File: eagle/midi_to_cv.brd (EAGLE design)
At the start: 100 x 80 mm, 57 parts, among them Q3 2N3904, Q4 2N3904, Q5 2N3904, Q6 2SK30, U1 ATMEGA328P_PDIP

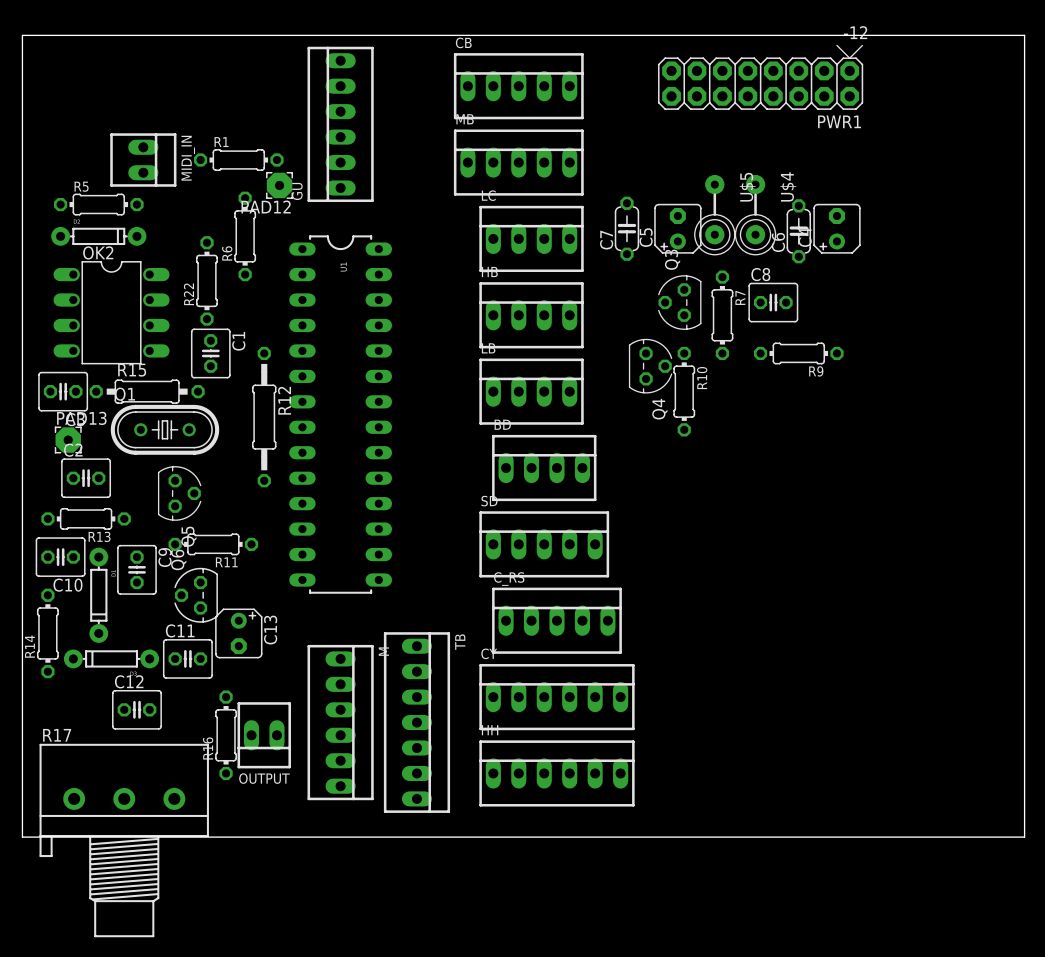
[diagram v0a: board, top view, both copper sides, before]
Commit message: 95pct auto
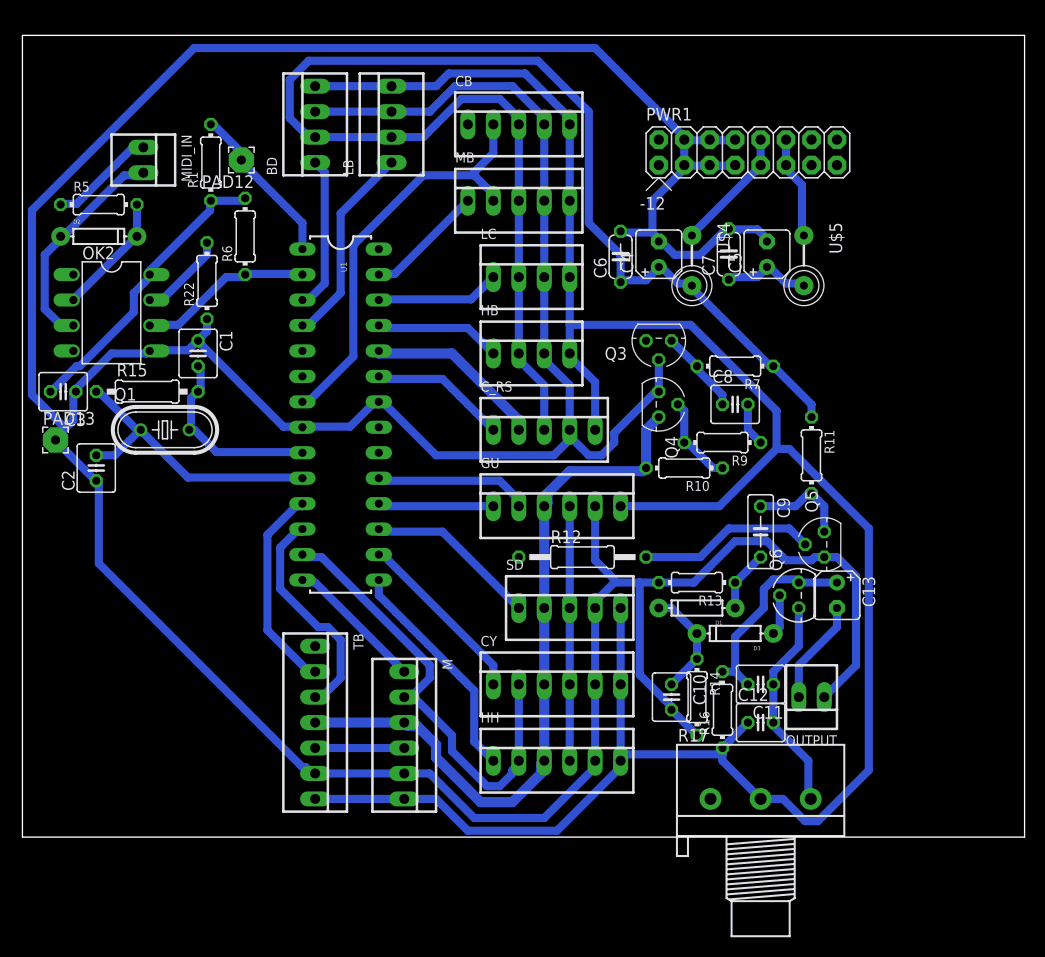
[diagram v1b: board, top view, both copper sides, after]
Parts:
- C9: device rcl:C025-040X050 -> rcl:C050-025X075
- moved R14 65.1 mm to (67.3, 14.0), turned to 270 degrees
- moved Q5 65.0 mm to (80.0, 29.2), turned to 90 degrees
- moved R17 63.5 mm to (73.7, 3.81)
- moved C10 62.5 mm to (64.8, 14.0), turned to 270 degrees
- moved C9 62.3 mm to (73.7, 30.5)
- moved D3 62.3 mm to (71.1, 20.3)
- moved C12 62.2 mm to (73.7, 11.4)
- moved R13 61.3 mm to (67.3, 25.4)
- moved R11 60.3 mm to (78.7, 38.1), turned to 270 degrees
- moved C13 59.8 mm to (81.3, 24.1)
- moved D1 59.7 mm to (67.3, 22.9), turned to 180 degrees
- moved Q6 59.7 mm to (77.5, 24.1)
- moved C11 57.2 mm to (73.7, 15.2), turned to 180 degrees
- moved OUTPUT 54.7 mm to (78.7, 14.0)
- moved R16 49.6 mm to (69.8, 12.7)
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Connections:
- removed net GU_LONG: GU.1, U1.3
- removed net GU_SHORT: GU.2, U1.4
- new net N$10: GU.2, U1.19
- new net N$9: GU.1, U1.18
- net ACCENT: now also U1.28; no longer U1.5
- net CB_TRIG: now also U1.5; no longer U1.28
- net CY_KILL: now also U1.13; no longer U1.14
- net C_TRIG: now also U1.24; no longer U1.18
- net M_TRIG: now also U1.14; no longer U1.13
- net N$3: now also U1.3; no longer U1.23
- net N$7: now also U1.4; no longer U1.24
- net RS_TRIG: now also U1.23; no longer U1.17
- net SD_TRIG: now also U1.17; no longer U1.19
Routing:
- net GND: track 0.00 -> 442.4 mm
- net RETURN: track 0.00 -> 227.4 mm
- net +12V: track 0.00 -> 174.4 mm
- net +5V: track 0.00 -> 80.8 mm
- net NOISE: track 0.00 -> 72.5 mm
- net CY_KILL: track 0.00 -> 47.1 mm
- net N$5: track 0.00 -> 29.7 mm
- net HH_TRIG: track 0.00 -> 22.8 mm
- net TB_KILL: track 0.00 -> 22.5 mm
- net N$17: track 0.00 -> 22.5 mm
- net N$29: track 0.00 -> 21.8 mm
- net TB_SHORT: track 0.00 -> 20.9 mm
- net N$32: track 0.00 -> 20.5 mm
- net N$7: track 0.00 -> 20.3 mm
- net N$4: track 0.00 -> 19.5 mm
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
